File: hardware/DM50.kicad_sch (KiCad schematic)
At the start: 111 parts, among them J1 ST-LINK, J2 USB_C_Receptacle_USB2.0_14P, J4 LiPO 3,7V, Q1 MMBT3904, SW1 SW_SPST, SW10 BT_SMD, SW11 BT_SMD, SW12 BT_SMD, SW13 BT_SMD, SW14 BT_SMD, SW15 BT_SMD, SW16 BT_SMD, SW17 BT_SMD, SW18 BT_SMD, SW19 BT_SMD, SW2 BT_SMD, SW20 BT_SMD, SW21 BT_SMD, SW22 BT_SMD, SW23 BT_SMD, SW24 BT_SMD, SW25 BT_SMD, SW26 BT_SMD, SW27 BT_SMD, SW28 BT_SMD, SW29 BT_SMD, SW3 BT_SMD, SW30 BT_SMD, SW31 BT_SMD, SW32 BT_SMD, SW33 BT_SMD, SW34 BT_SMD, SW35 BT_SMD, SW36 BT_SMD, SW37 BT_SMD, SW38 BT_SMD, SW39 BT_SMD, SW4 BT_SMD, SW40 BT_SMD, SW41 BT_SMD, SW42 SW_SPST, SW43 BT_SMD, SW44 BT_SMD, SW45 BT_SMD, SW46 BT_SMD, SW47 BT_SMD, SW48 BT_SMD, SW49 BT_SMD, SW5 BT_SMD, SW50 BT_SMD, SW51 BT_SMD, SW52 BT_SMD, SW6 BT_SMD, SW7 BT_SMD, SW8 BT_SMD, SW9 BT_SMD, U1 EA_DOGL128X-6, U2 STM32U575RIT6, U3 W25Q128JVSIQ, U4 USBLC6-2SC6, U5 ADP2108AUJ-3.3, U6 MCP73831, Y1 32768

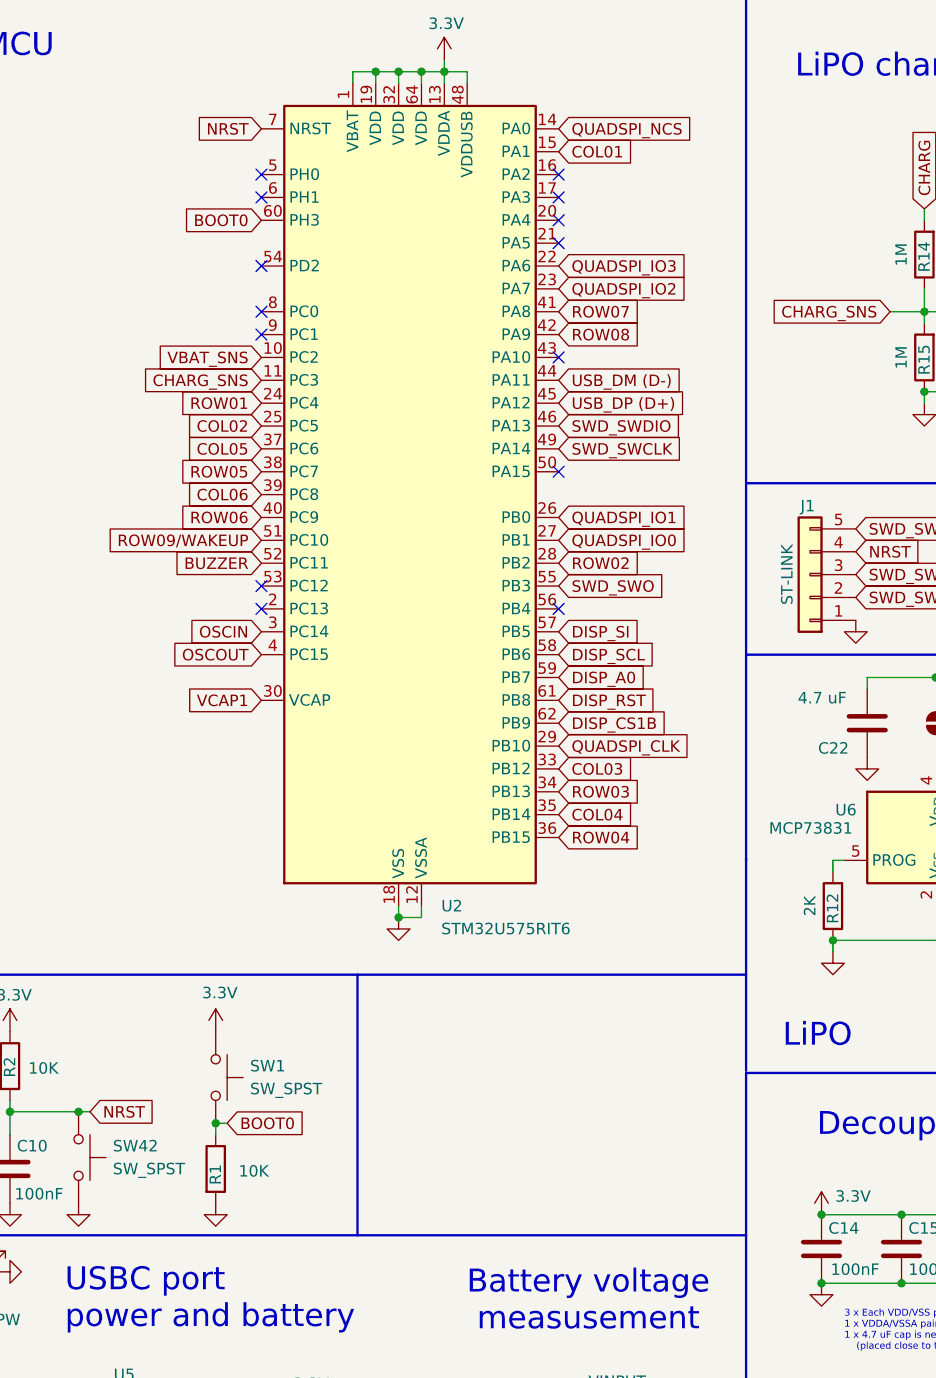
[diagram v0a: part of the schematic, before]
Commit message: PCB CHANGES
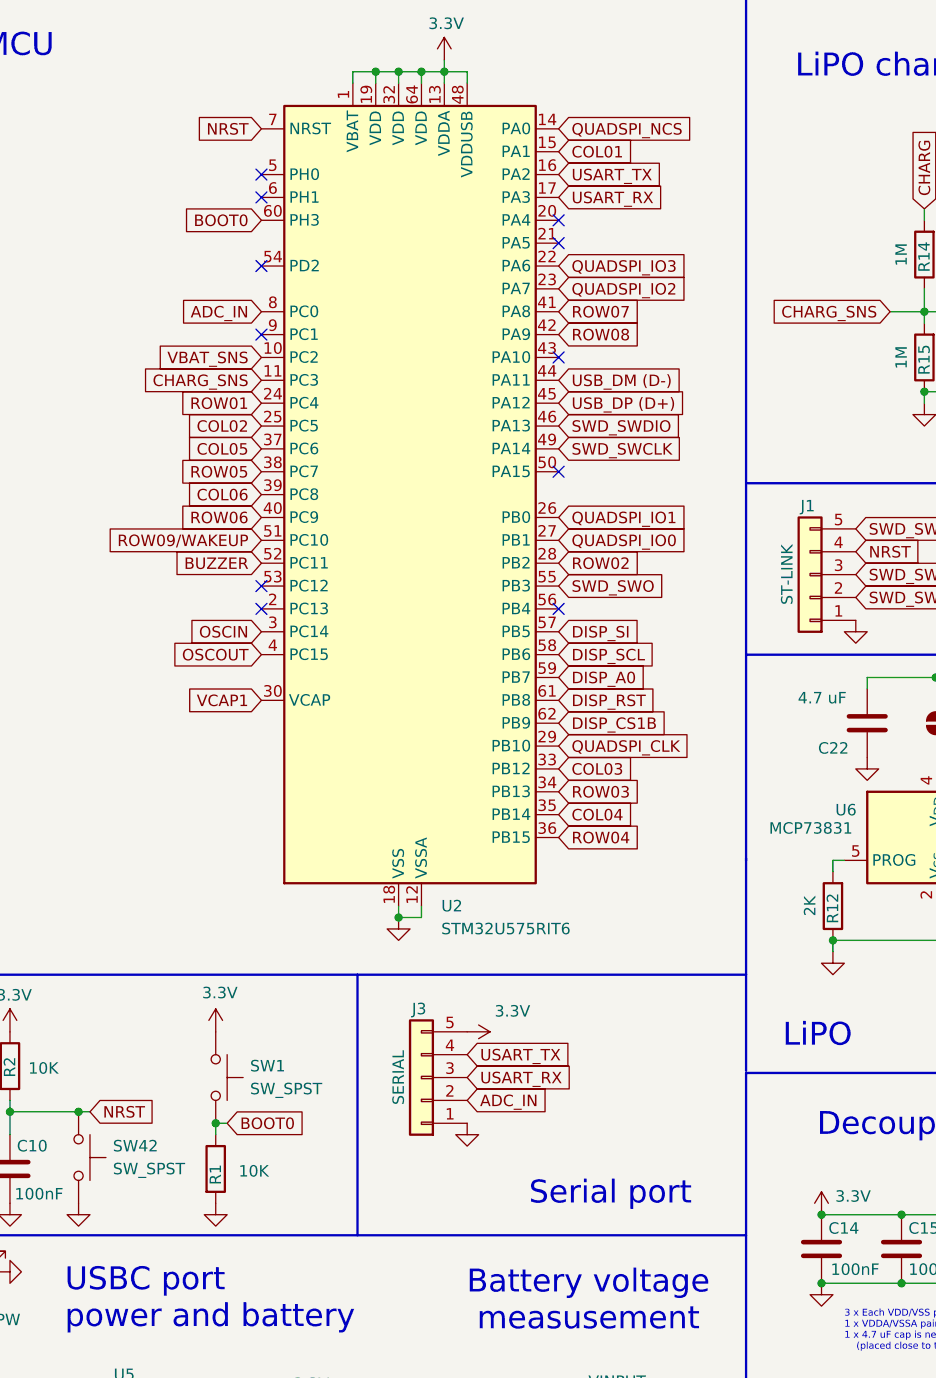
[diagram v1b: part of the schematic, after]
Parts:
- added J3: SERIAL, DM50:SAMTEC-SMH-105-02-X-S, symbol Connector_Generic:Conn_01x05
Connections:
- net 3.3V: now also J3.5 (Pin_5)
- net GND: now also J3.1 (Pin_1)
- net USART_TX: now reaches U2.16 (PA2)
- net USART_TX: now also J3.4 (Pin_4)
- net USART_RX: now reaches U2.17 (PA3)
- net USART_RX: now also J3.3 (Pin_3)
- net ADC_IN: now reaches U2.8 (PC0)
- net ADC_IN: now also J3.2 (Pin_2)
- no-connect marks 20 -> 17
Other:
- note added: "Serial port"
